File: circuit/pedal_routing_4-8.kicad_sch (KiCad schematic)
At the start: 4 parts, among them U115 CD4051B, U117 CD4051B, U118 CD4051B, U120 CD4051B

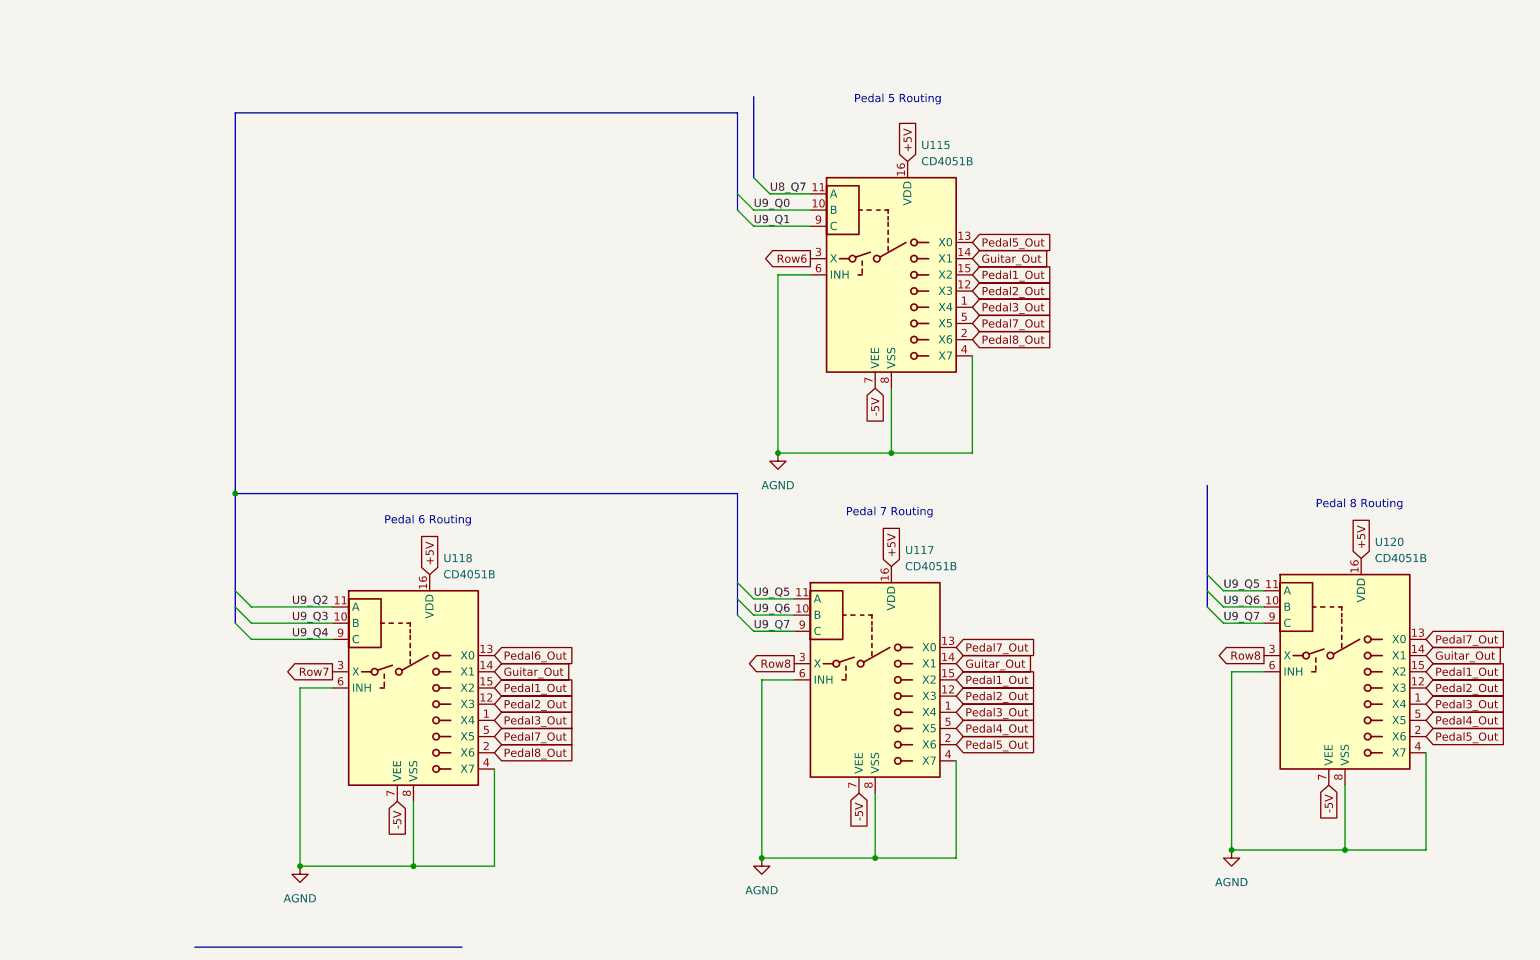
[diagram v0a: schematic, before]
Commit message: Rebuilt bus and matrix.
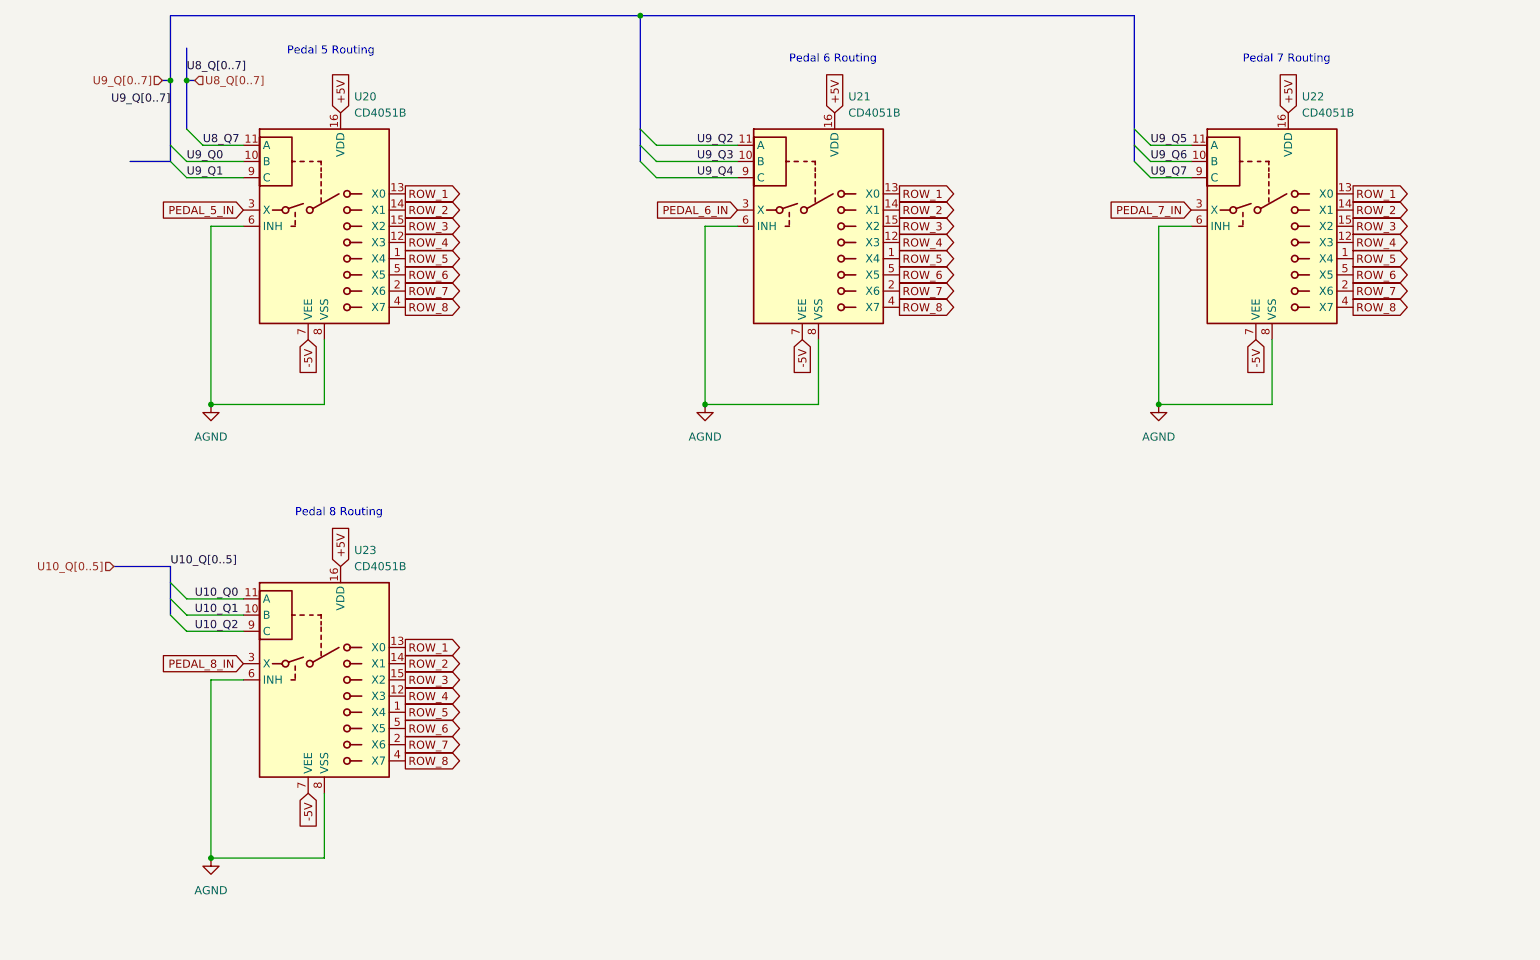
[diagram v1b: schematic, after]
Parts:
- renumbered U115 to U20, U118 to U21, U117 to U22, U120 to U23
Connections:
- net Pedal8_Out is gone; now on net ROW_7: U20.2 (X6), U21.2 (X6)
- net AGND: no longer U20.4 (X7), U21.4 (X7), U22.4 (X7), U23.4 (X7)
- net U9_Q5: no longer U23.11 (A)
- net U9_Q6: no longer U23.10 (B)
- net U9_Q7: no longer U23.9 (C)
- net Guitar_Out renamed ROW_2
- net Pedal1_Out renamed ROW_3
- net Pedal2_Out renamed ROW_4
- net Pedal3_Out renamed ROW_5
- net Pedal4_Out renamed ROW_6
- net ROW_6: now also U20.5 (X5), U21.5 (X5)
- net Pedal5_Out renamed ROW_7
- net ROW_7: no longer U20.13 (X0)
- net Pedal6_Out renamed ROW_1
- net ROW_1: now also U20.13 (X0), U22.13 (X0), U23.13 (X0)
- removed net Pedal7_Out: U20.5 (X5), U21.5 (X5), U22.13 (X0), U23.13 (X0)
- net Row6 renamed PEDAL_5_IN
- net Row7 renamed PEDAL_6_IN
- net Row8 renamed PEDAL_7_IN
- net PEDAL_7_IN: no longer U23.3 (X)
- new net PEDAL_8_IN: U23.3 (X)
- new net ROW_8: U20.4 (X7), U21.4 (X7), U22.4 (X7), U23.4 (X7)
- new net U10_Q0: U23.11 (A)
- new net U10_Q1: U23.10 (B)
- new net U10_Q2: U23.9 (C)
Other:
- moved on the sheet: U20, U21, U22, U23
